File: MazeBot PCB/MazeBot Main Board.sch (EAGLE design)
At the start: 14 parts, among them IC1 7805TV, IC2 L298

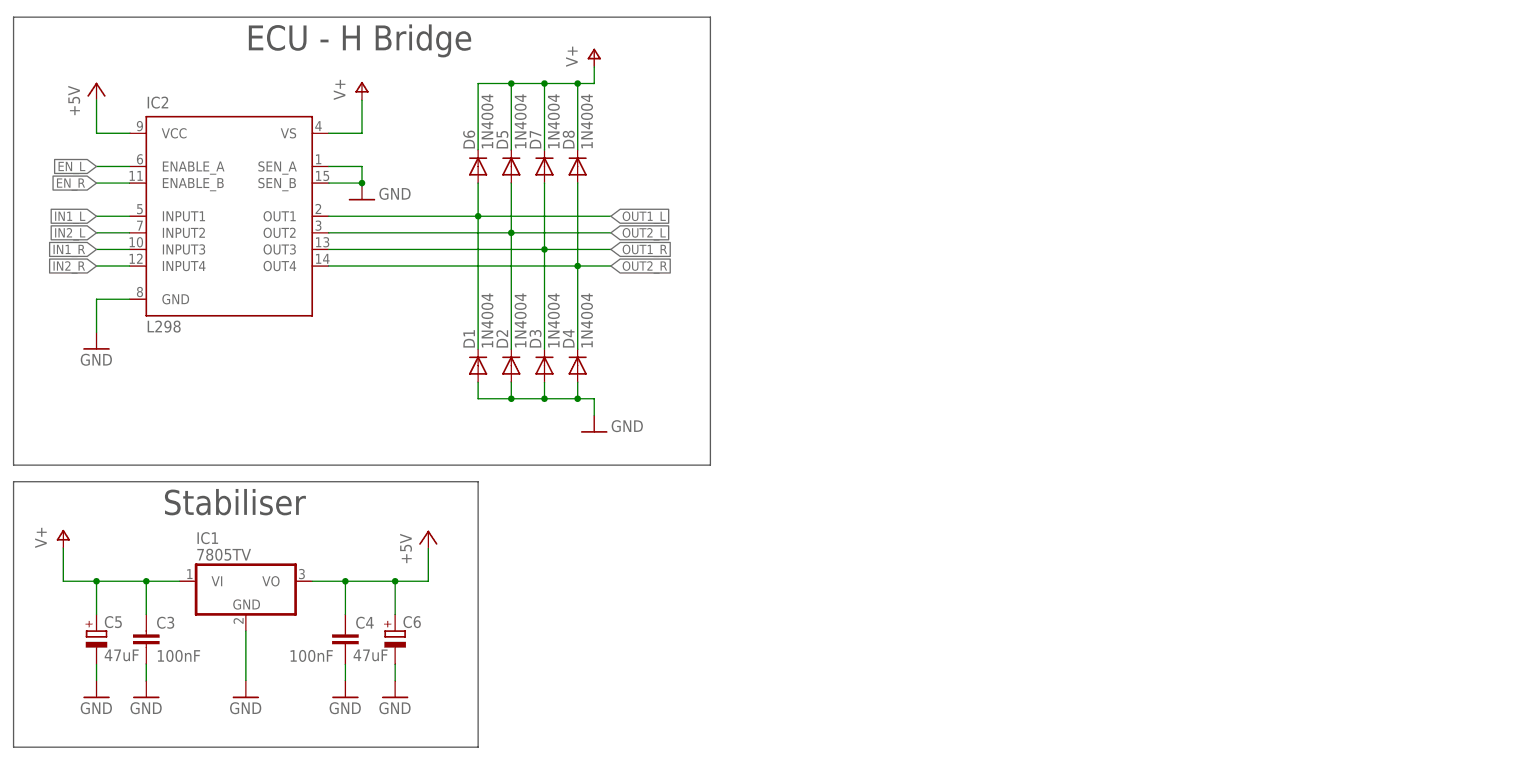
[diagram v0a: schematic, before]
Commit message: Add ATMEGA with XTAL
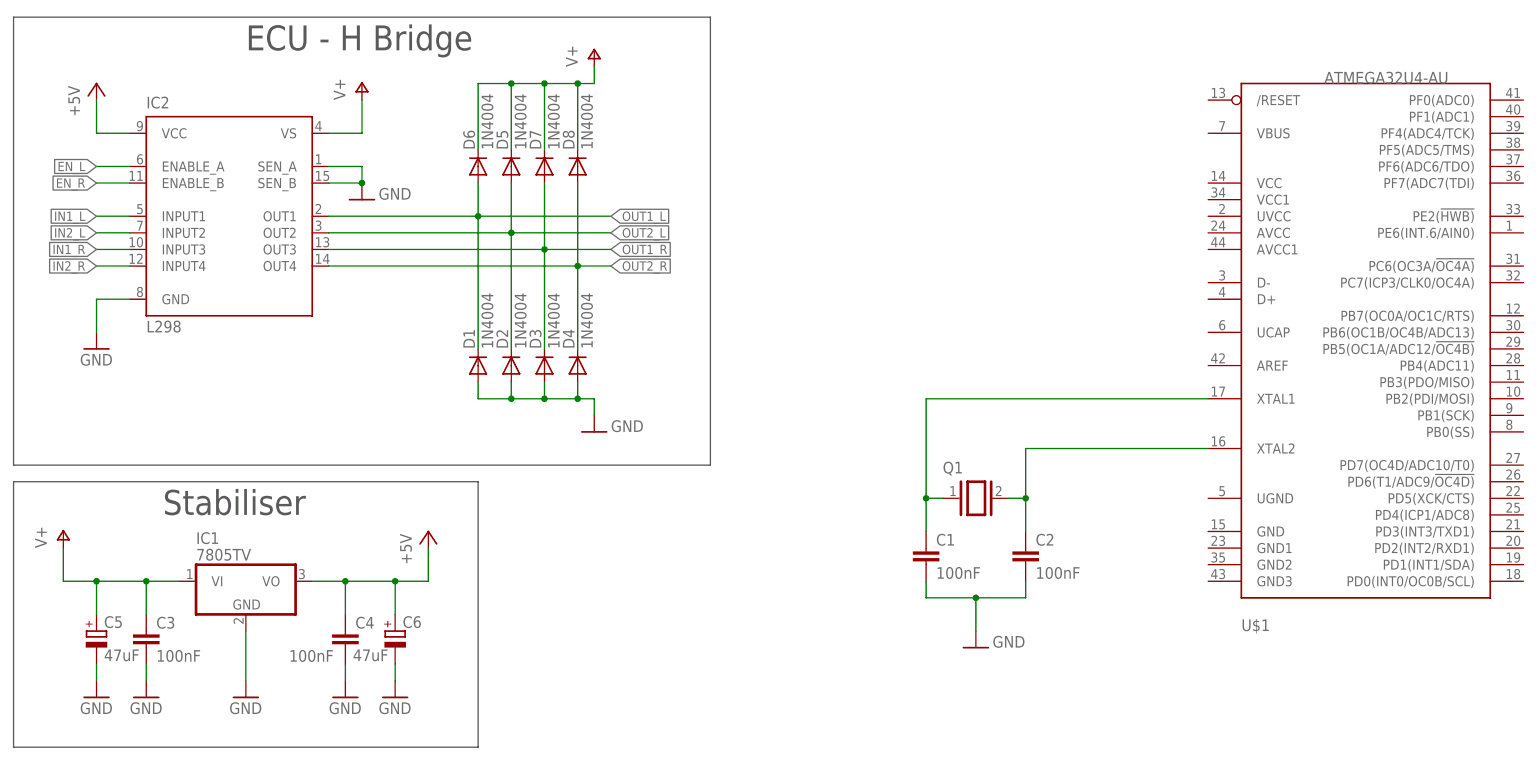
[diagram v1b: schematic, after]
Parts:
- added C1, C2: 100nF, rcl:C-EU025-024X044
- added Q1: (no value), special:XTAL/S
- added U$1: ATMEGA32U4-AU, adafruit:ATMEGA32U4-AU
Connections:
- new net N$1: C1.1, Q1.1, U$1.XTAL1
- new net N$2: C2.1, Q1.2, U$1.XTAL2
- net GND: now also C1.2, C2.2
